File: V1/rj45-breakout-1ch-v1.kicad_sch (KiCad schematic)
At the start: 2 parts, among them J1 RJ45, J2 1x4P 5,08 SCREW

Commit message: Update board title
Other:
- title: 1 channel RJ45 breakout board -> 1 Channel RJ45 Breakout Board
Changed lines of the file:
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@@
 	(paper "A4")
 	(title_block
-		(title "1 channel RJ45 breakout board")
+		(title "1 Channel RJ45 Breakout Board")
 		(date "2022-04-01")
 		(rev "V1")

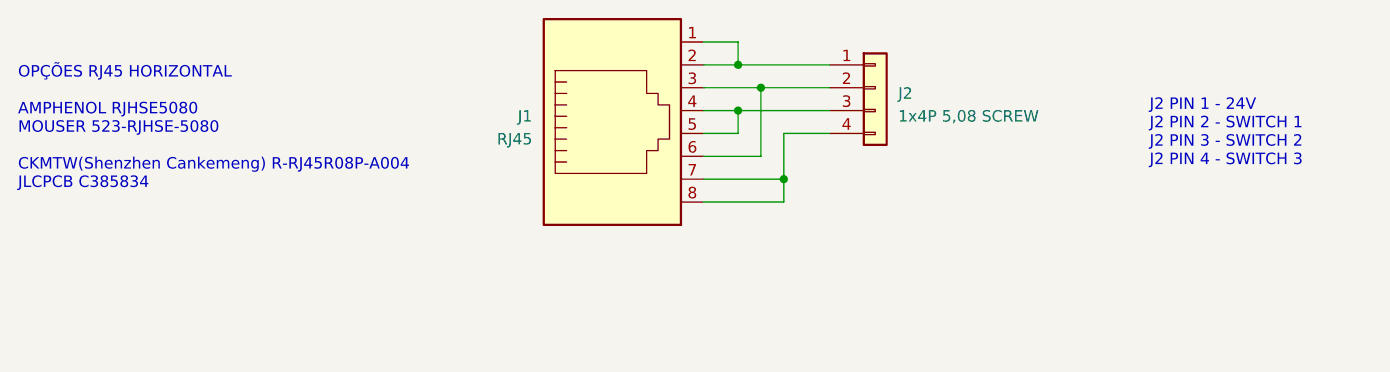
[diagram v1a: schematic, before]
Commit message: Revising before manufacturing
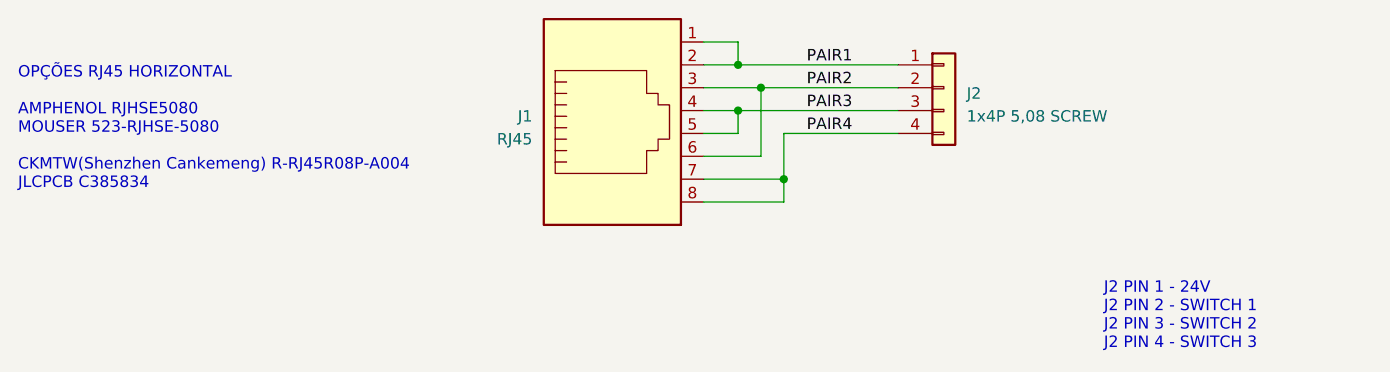
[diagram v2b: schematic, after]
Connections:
- net PAIR1: now reaches J1.1, J1.2, J2.1 (Pin_1)
- net PAIR2: now reaches J1.3, J1.6, J2.2 (Pin_2)
- net PAIR3: now reaches J1.4, J1.5, J2.3 (Pin_3)
- net PAIR4: now reaches J1.7, J1.8, J2.4 (Pin_4)
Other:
- moved on the sheet: J2
